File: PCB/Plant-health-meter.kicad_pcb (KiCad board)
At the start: 4 copper layers, 136.2 x 25 mm, 91 parts, among them J1 Conn_01x02, J2 Conn_01x02, J3 Conn_01x04, J4 UJ2-MIBH2-4-SMT-TR, J5 Conn_01x02, Q1 AO3401A, SW1 Boot, SW2 Reset, U1 LTC4412xS6, U12 ADS1115IDGS, U2 TPS62172DSG, U3 USBLC6-2P6, U4 ESP32-C3FH4X, U5 BME280, U6 TPS61022, U7 OPA340NA, U8 TP4057, U9 TLC555xD, Y1 40MHz

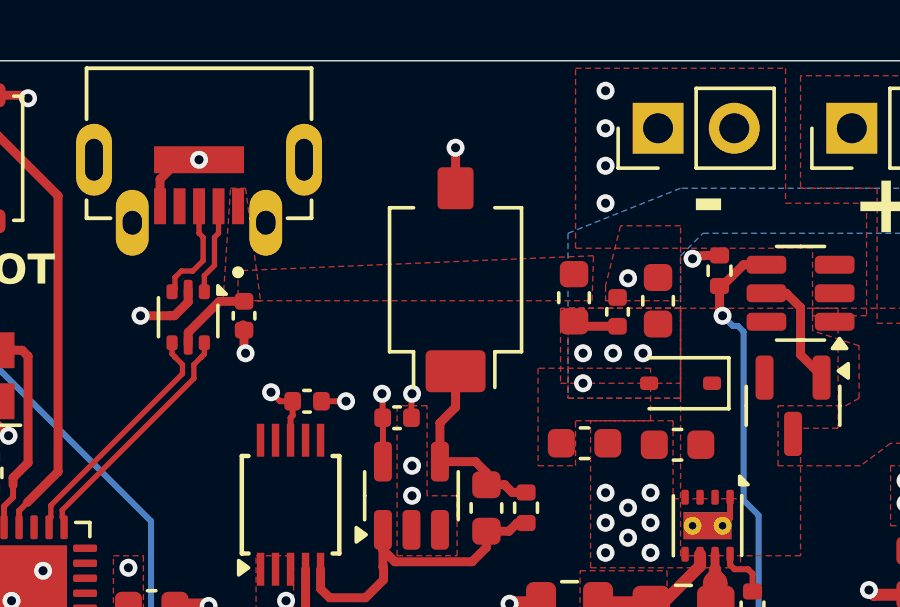
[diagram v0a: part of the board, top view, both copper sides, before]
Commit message: Light sensor
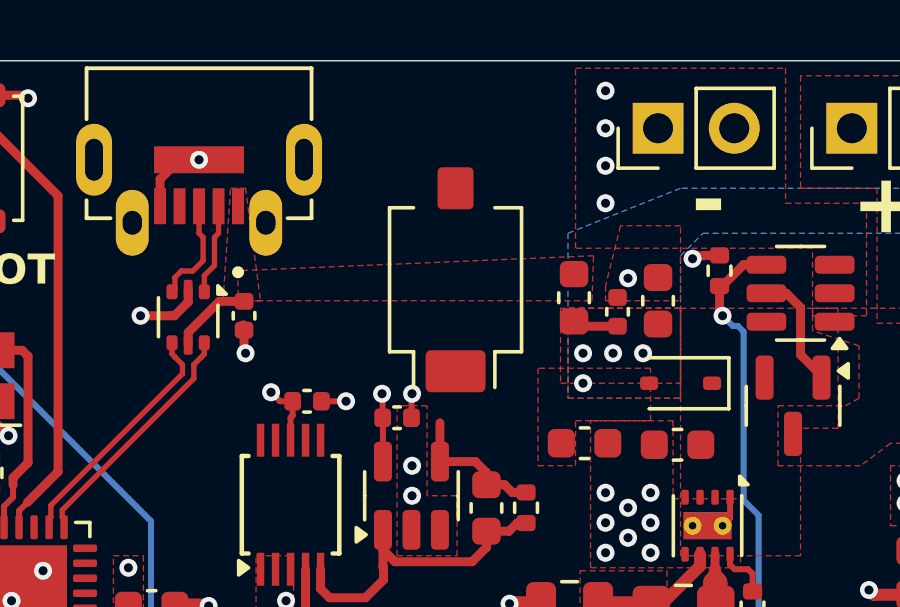
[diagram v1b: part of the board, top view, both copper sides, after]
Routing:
- net Net-(D7-K): track 6.76 -> 4.82 mm
- net GND: track 44.0 -> 42.6 mm, vias 108 -> 107
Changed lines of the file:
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@@
 			(outputformat 1)
 			(mirror no)
-			(drillshape 1)
+			(drillshape 0)
 			(scaleselection 1)
-			(outputdirectory "")
+			(outputdirectory "manufacture/")
 		)
 	)
@@
 		(tags "capacitor")
 		(property "Reference" "C31"
-			(at 0 -1.16 360)
+			(at 0 -1.16 0)
 			(layer "F.SilkS")
 			(hide yes)
@@
 		)
 		(property "Value" "100n"
-			(at 0 1.16 360)
+			(at 0 1.16 0)
 			(layer "F.Fab")
 			(effects
@@
 		)
 		(fp_text user "${REFERENCE}"
-			(at 0 0 360)
+			(at 0 0 0)
 			(layer "F.Fab")
 			(effects
@@
 		(tags "capacitor")
 		(property "Reference" "C1"
-			(at 0 -1.16 360)
+			(at 0 -1.16 0)
 			(layer "F.SilkS")
 			(hide yes)
@@
 		)
 		(property "Value" "100n"
-			(at 0 1.16 360)
+			(at 0 1.16 0)
 			(layer "F.Fab")
 			(effects
@@
 		)
 		(fp_text user "${REFERENCE}"
-			(at 0 0 360)
+			(at 0 0 0)
 			(layer "F.Fab")
 			(effects
@@
 	)
 	(segment
-		(start 123 101.75)
-		(end 123 100.4)
-		(width 0.3)
-		(layer "F.Cu")
-		(net 2)
-	)
-	(segment
 		(start 115.95 106.48)
 		(end 115.95 107.2)
@@
 	)
 	(via
-		(at 123 100.4)
-		(size 0.6)
-		(drill 0.3)
-		(layers "F.Cu" "B.Cu")
-		(net 2)
-	)
-	(via
 		(at 91.75 110)
 		(size 0.6)
@@
 	)
 	(segment
-		(start 122.479999 109.57)
-		(end 123 109.049999)
-		(width 0.3)
-		(layer "F.Cu")
-		(net 57)
-	)
-	(segment
 		(start 124.6325 111.6325)
 		(end 124.029999 111.6325)
@@
 		(width 0.3)
 		(layer "F.Cu")
-		(net 57)
-	)
-	(segment
-		(start 123 109.049999)
-		(end 123 107.85)
-		(width 0.3)
-		(layer "F.Cu")

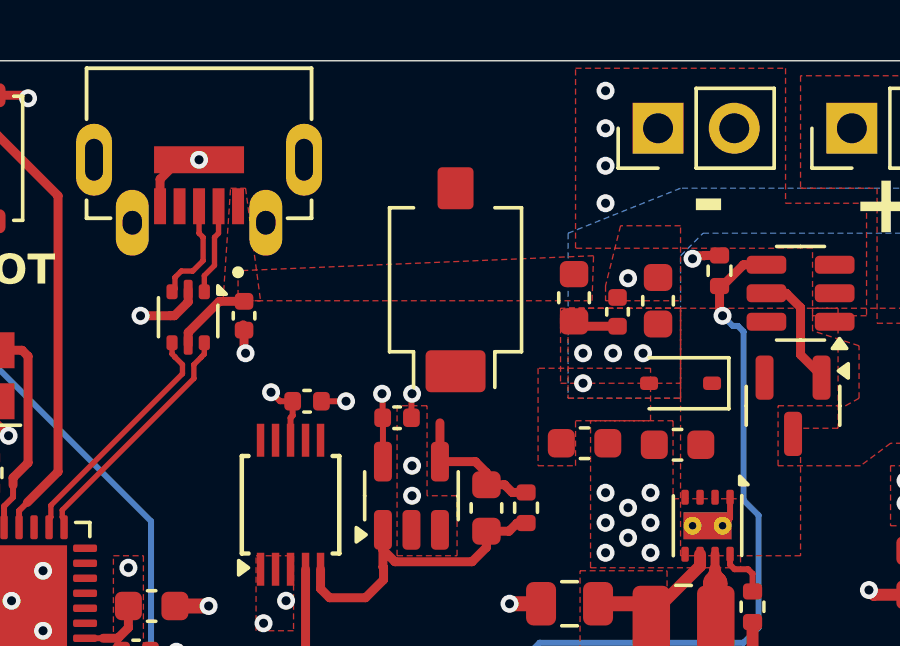
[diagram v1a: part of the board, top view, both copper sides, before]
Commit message: Cleaned up
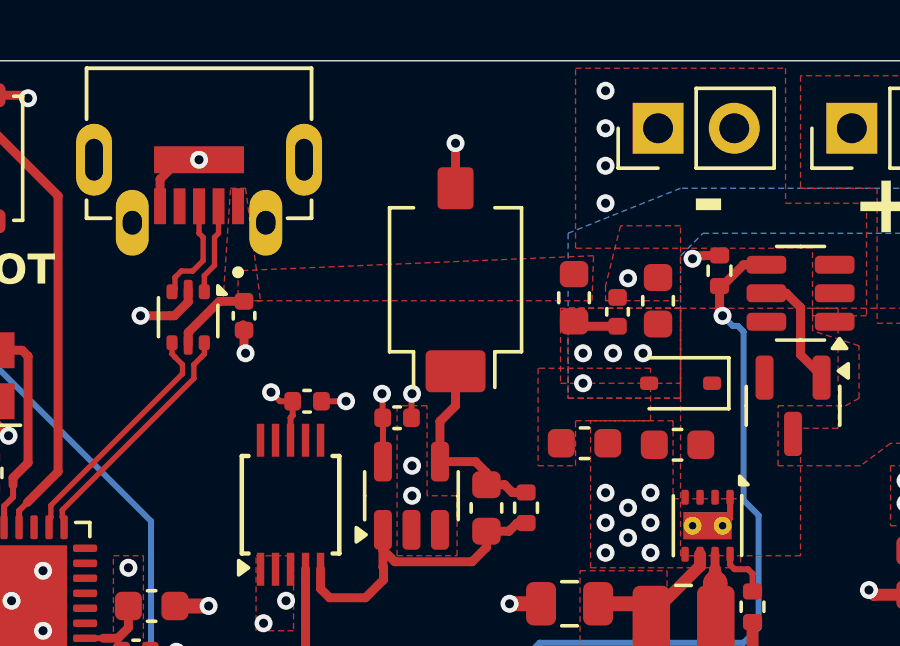
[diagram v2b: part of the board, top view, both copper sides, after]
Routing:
- net Net-(D7-K): track 4.82 -> 6.76 mm
- net GND: track 42.6 -> 44.1 mm, vias 107 -> 108
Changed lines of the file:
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@@
 	)
 	(segment
+		(start 123 101.75)
+		(end 123 100.25)
+		(width 0.3)
+		(layer "F.Cu")
+		(net 2)
+	)
+	(segment
 		(start 138.69 116.6)
 		(end 138.3975 116.8925)
@@
 	)
 	(via
+		(at 123 100.25)
+		(size 0.6)
+		(drill 0.3)
+		(layers "F.Cu" "B.Cu")
+		(net 2)
+	)
+	(via
 		(at 94.5 98.75)
 		(size 0.6)
@@
 	)
 	(segment
-		(start 124.89 111.89)
-		(end 124.6325 111.6325)
+		(start 122.479999 109.520001)
+		(end 123 109)
 		(width 0.3)
 		(layer "F.Cu")
@@
 	)
 	(segment
-		(start 124.029999 111.229999)
-		(end 124.029999 111.6325)
+		(start 123 109)
+		(end 123 107.85)
 		(width 0.3)
 		(layer "F.Cu")
@@
 	(segment
 		(start 122.479999 110.8625)
-		(end 122.479999 109.57)
+		(end 122.479999 109.520001)
+		(width 0.3)
+		(layer "F.Cu")
+		(net 57)
+	)
+	(segment
+		(start 124.89 111.89)
+		(end 124.6325 111.6325)
+		(width 0.3)
+		(layer "F.Cu")
+		(net 57)
+	)
+	(segment
+		(start 124.029999 111.229999)
+		(end 124.029999 111.6325)
 		(width 0.3)
 		(layer "F.Cu")
